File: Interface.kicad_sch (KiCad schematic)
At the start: 20 parts, among them J1 Debugger, J2 USART, J3 SPI, J4 USB_C_Receptacle_USB2.0, Q1 Q_NMOS_GSD, U3 USBLC6-2SC6

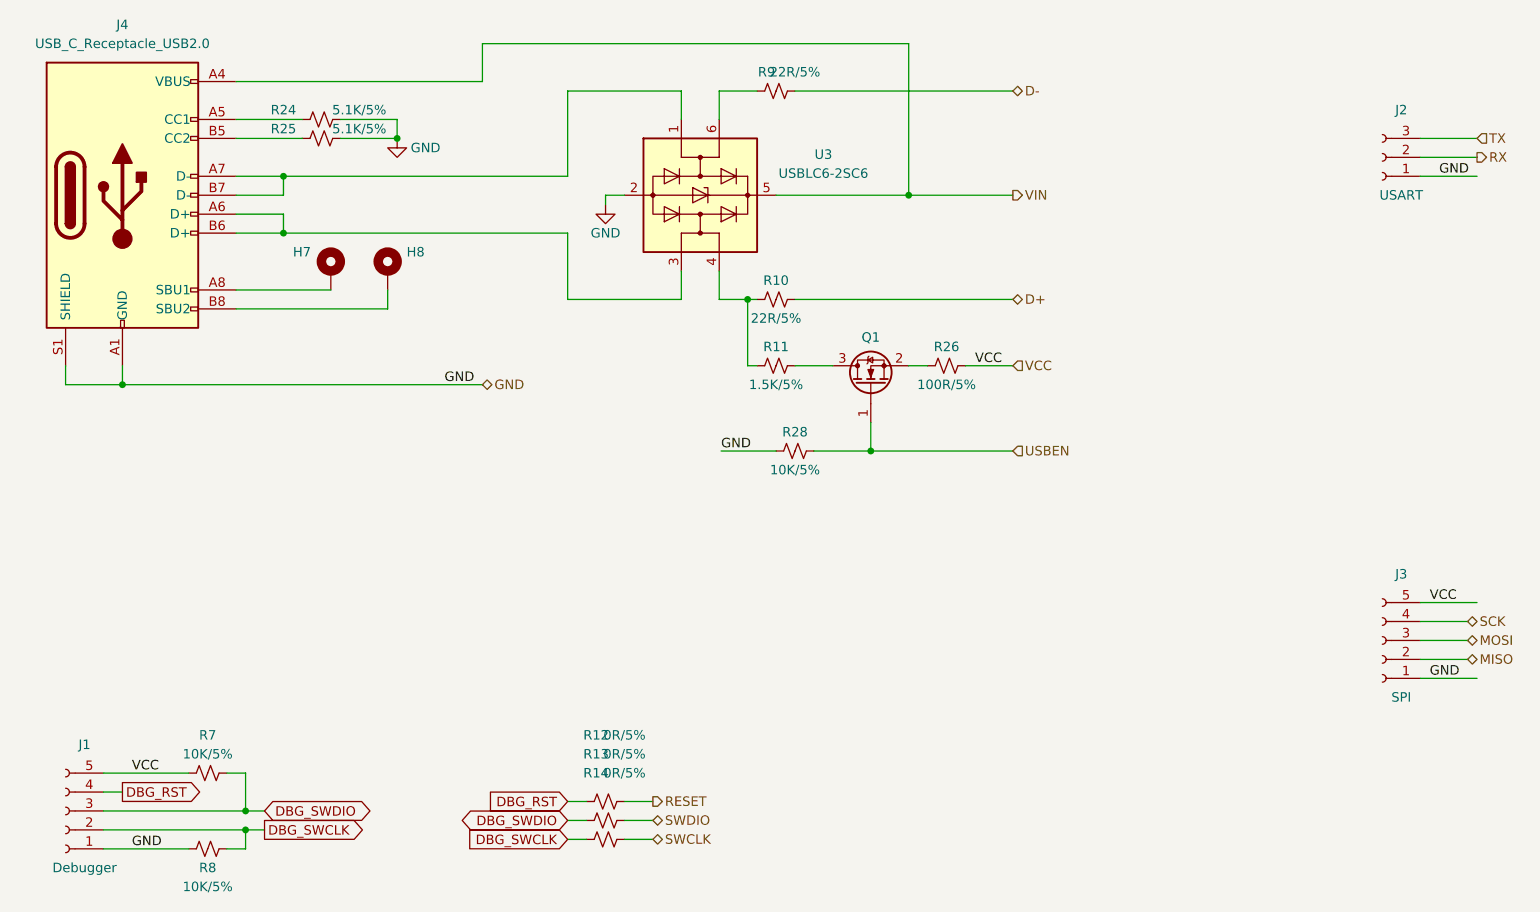
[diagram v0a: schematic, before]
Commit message: update pcb layout
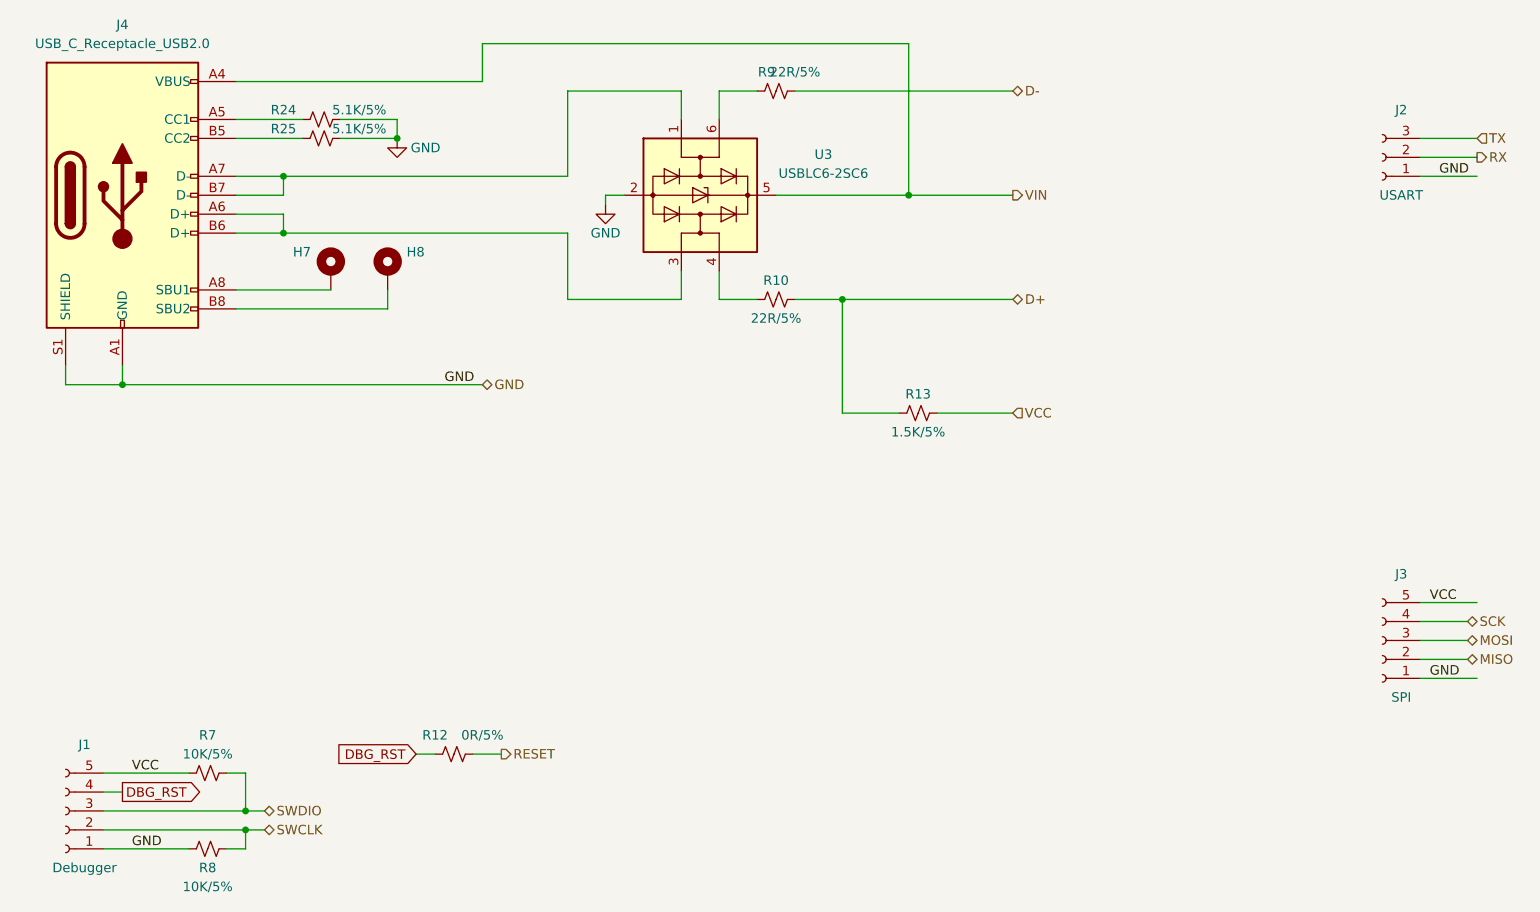
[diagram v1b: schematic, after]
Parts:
- removed Q1: Q_NMOS_GSD, Package_TO_SOT_SMD:SOT-23, symbol Device:Q_NMOS_GSD
- removed R11: 1.5K/5%, Resistor_SMD:R_0603_1608Metric, symbol Device:R_Small_US
- removed R14: 0R/5%, Resistor_SMD:R_0603_1608Metric, symbol Device:R_Small_US
- removed R26: 100R/5%, Resistor_SMD:R_0603_1608Metric, symbol Device:R_Small_US
- removed R28: 10K/5%, Resistor_SMD:R_0603_1608Metric, symbol Device:R_Small_US
- R13: value 0R/5% -> 1.5K/5%
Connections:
- net DBG_SWCLK is gone; now on net SWCLK: J1.2 (Pin_2), R8.2
- net D+: now also R13.1
- net SWDIO: now also J1.3 (Pin_3), R7.2; no longer R13.2
- net VCC: now also R13.2
- removed net DBG_SWDIO: J1.3 (Pin_3), R13.1, R7.2
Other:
- moved on the sheet: R12
